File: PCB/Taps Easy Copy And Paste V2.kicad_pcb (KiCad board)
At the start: 2 copper layers, 42.9 x 83.3 mm, 7 parts, among them SW1 SW_Push, SW2 SW_Push, SW3 SW_Push, SW4 SW_Push, U1 XIAO HERE, U2 OLED_0.91_I2C

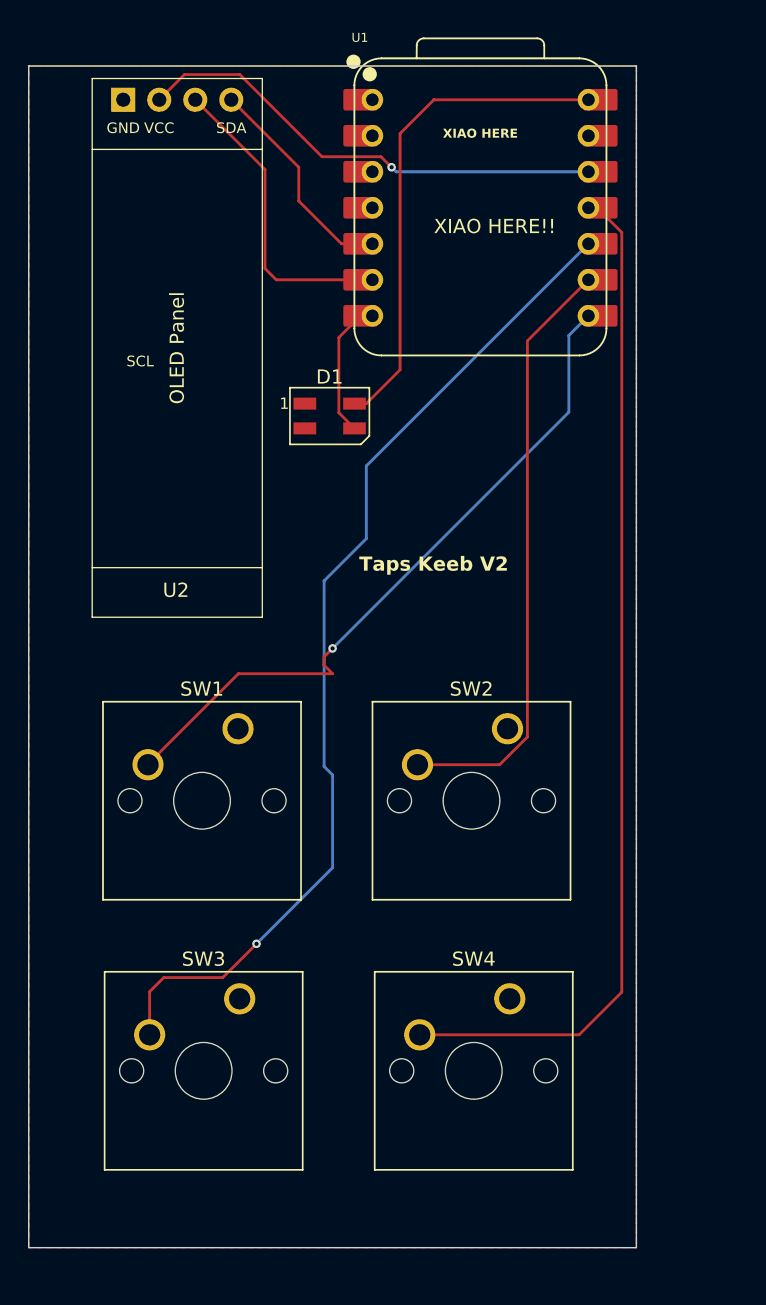
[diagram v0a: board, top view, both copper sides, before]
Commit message: Add files via upload
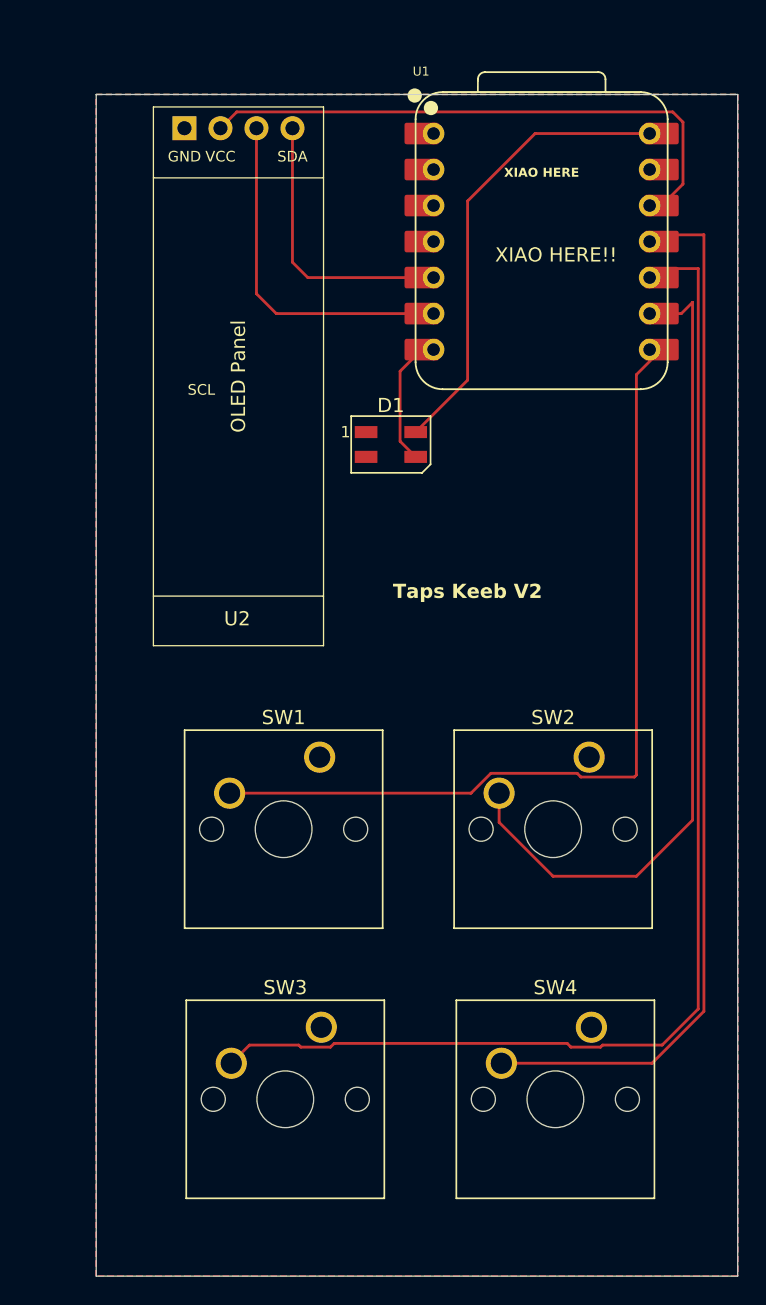
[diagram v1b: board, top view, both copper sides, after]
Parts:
- moved SW1 6.10 mm to (34.8, 63.0)
- moved SW2 6.10 mm to (53.8, 63.0)
- moved SW4 6.10 mm to (54.0, 82.1)
- moved SW3 6.10 mm to (34.9, 82.1)
- moved U1 4.93 mm to (50.5, 26.7)
- moved D1 4.76 mm to (39.8, 41.0)
- moved U2 4.76 mm to (23.1, 55.2)
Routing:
- net Net-(U1-GPIO4/MISO): track 71.5 -> 89.9 mm, vias 1 -> 0
- net Net-(U1-GPIO2/SCK): track 42.6 -> 58.0 mm
- net Net-(U1-GPIO1/RX): track 48.9 -> 60.2 mm, vias 1 -> 0
- net Net-(U1-3V3): track 33.9 -> 39.9 mm, vias 1 -> 0
- net Net-(U1-GPIO6/SDA): track 15.6 -> 19.0 mm
- net +5V: track 35.1 -> 32.6 mm
- net Net-(U1-GPIO7/SCL): track 21.8 -> 23.9 mm
- net Net-(U1-GPIO3/MOSI): track 72.2 -> 73.8 mm
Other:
- board size 42.9 x 83.3 mm -> 45.2 x 83.3 mm
